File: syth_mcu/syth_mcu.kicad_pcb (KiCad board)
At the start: 2 copper layers, 100 x 100 mm, 56 parts, among them J1 Conn_01x05, J2 Conn_01x05, J3 USB_C_Receptacle_PowerOnly_6P, J4 AudioPlug3, J5 Conn_01x20, J6 Conn_01x20, J7 Conn_01x16, J8 Conn_01x08, J9 Conn_01x07, Q1 SI2307DS, Q2 SI2304DS, Q3 SI2307DS, Q4 SI2304DS, SW1 SW_Push, SW2 SW_Push, SW3 SW_Push, SW4 SW_Push, SW5 SW_Push, U2 YAAJ_WeAct_BlackPill_Part_Like, U3 AMS1117-3.3, U4 AMS1117-3.3, U5 TFT_320x240

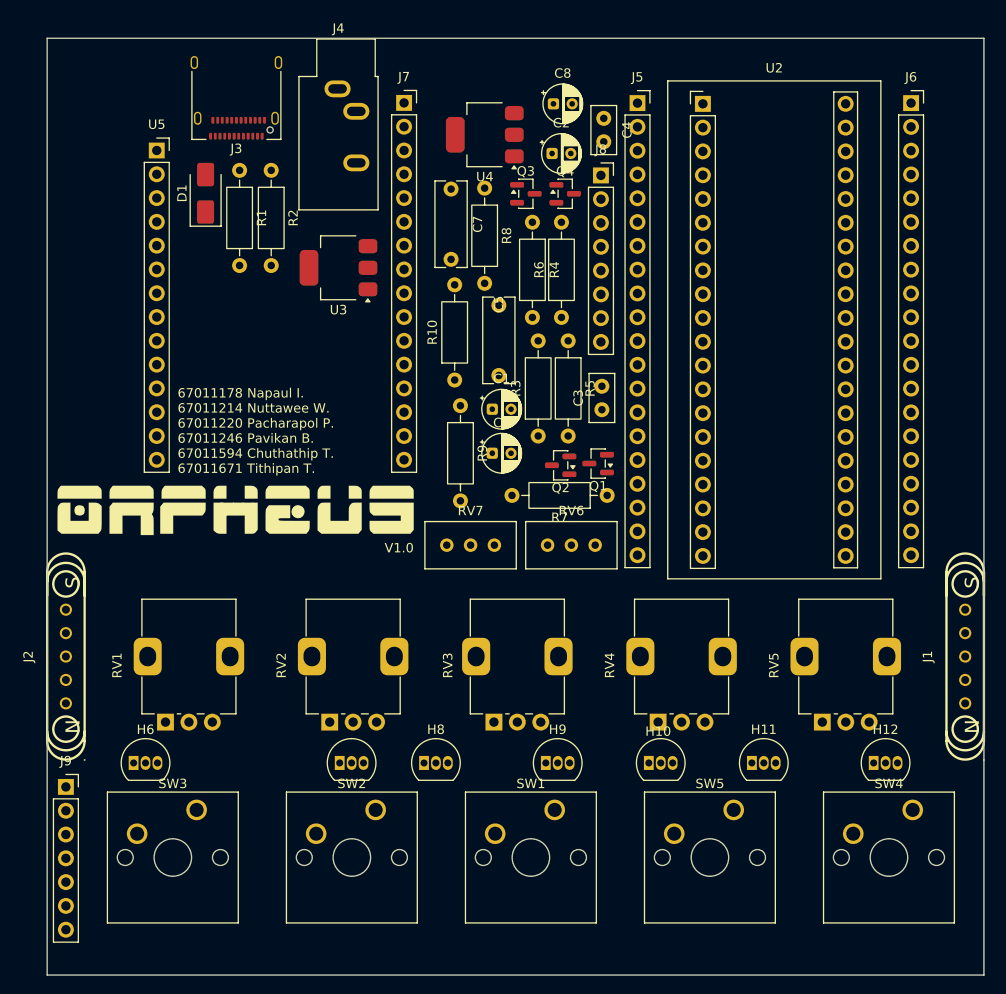
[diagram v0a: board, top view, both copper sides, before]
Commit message: update layout
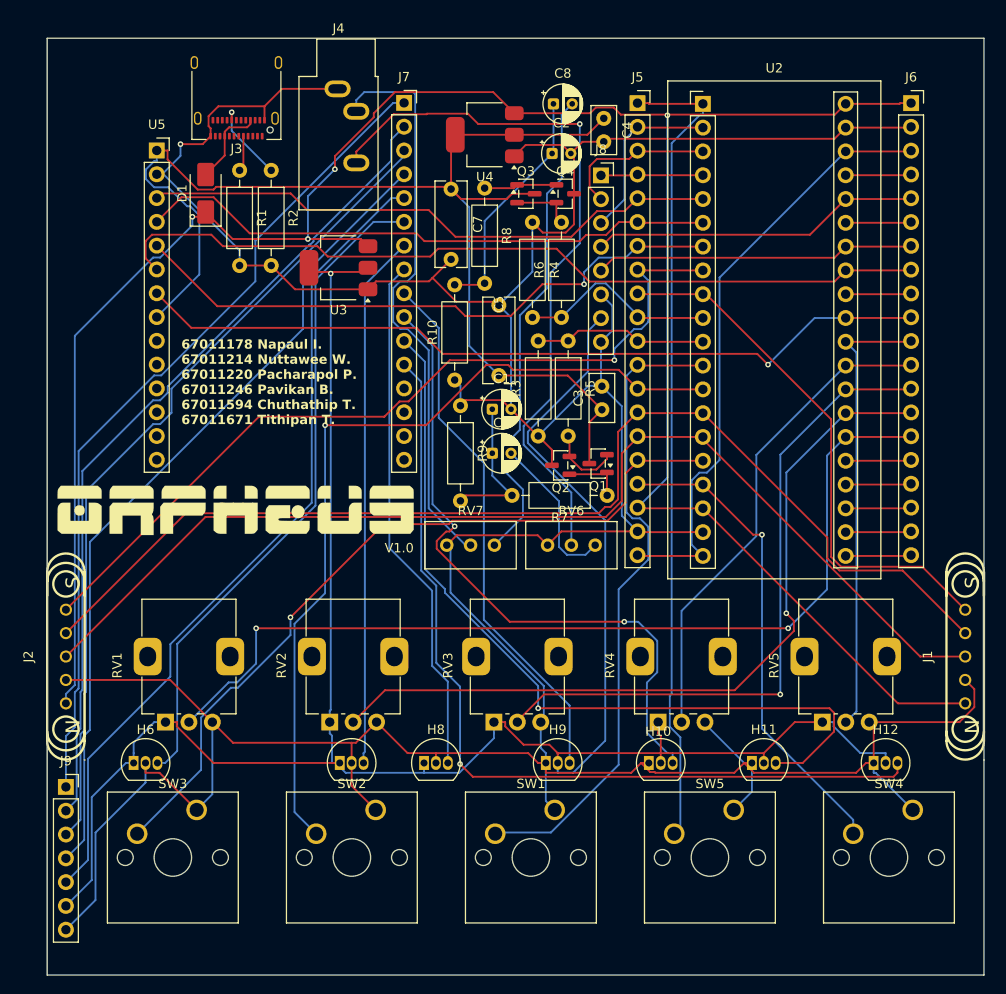
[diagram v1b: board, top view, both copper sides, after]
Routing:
- net ENN: track 0.00 -> 453.4 mm, vias 0 -> 1
- net D_5V: track 0.00 -> 242.0 mm, vias 0 -> 4
- net AMS1_3.3V: track 0.00 -> 240.9 mm, vias 0 -> 1
- net AMS2_3.3V: track 0.00 -> 130.5 mm
- net PB6: track 0.00 -> 121.0 mm
- net PB7: track 0.00 -> 118.6 mm
- net PA0: track 0.00 -> 100.3 mm, vias 0 -> 2
- net C11: track 0.00 -> 93.6 mm, vias 0 -> 1
- net PB5: track 0.00 -> 90.0 mm, vias 0 -> 1
- net C0: track 0.00 -> 89.1 mm
- net PA7: track 0.00 -> 88.8 mm
- net C4: track 0.00 -> 88.8 mm
- net PA11: track 0.00 -> 88.7 mm, vias 0 -> 1
- net C1: track 0.00 -> 88.5 mm
- net C2: track 0.00 -> 88.4 mm
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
